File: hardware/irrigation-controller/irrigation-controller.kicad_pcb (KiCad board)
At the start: 2 copper layers, 109 x 48.3 mm, 39 parts, among them J1 RS485, J12 RELAY_2, J3 I/O, J5 RF Module, J6 PWR 24V, J7 RELAY_1, J8 ESP32, J9 ESP32, U1 AQY280EH, U3 AQY280EH, U4 TPS54331DR, U6 MAX3485

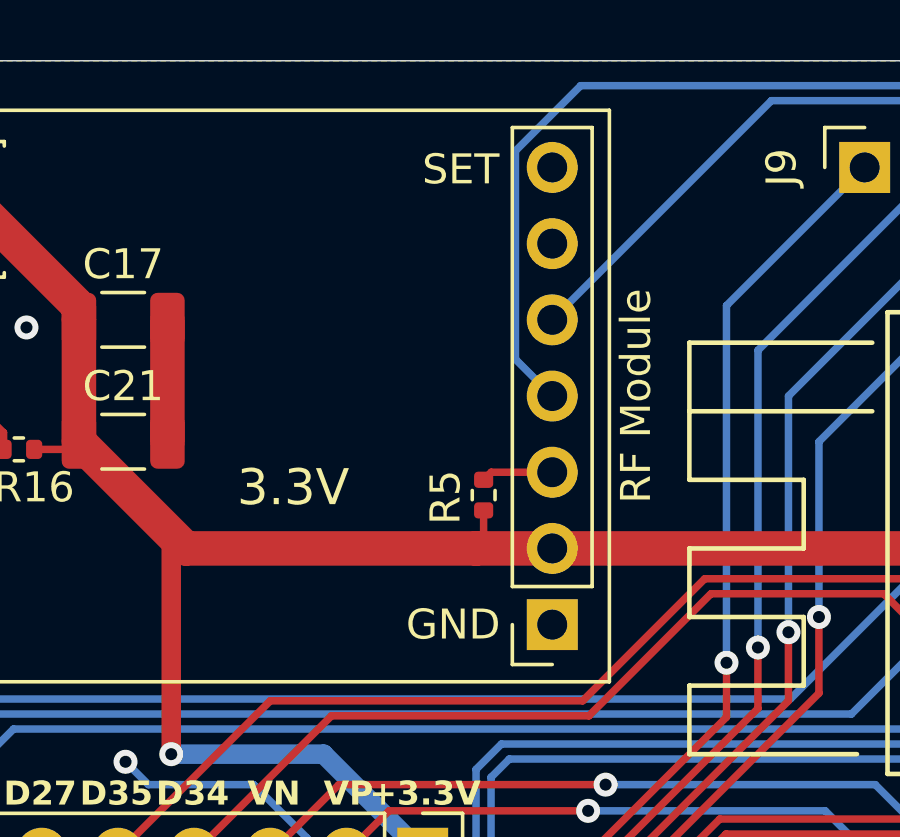
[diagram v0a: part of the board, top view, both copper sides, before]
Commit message: Update remote unit PCB
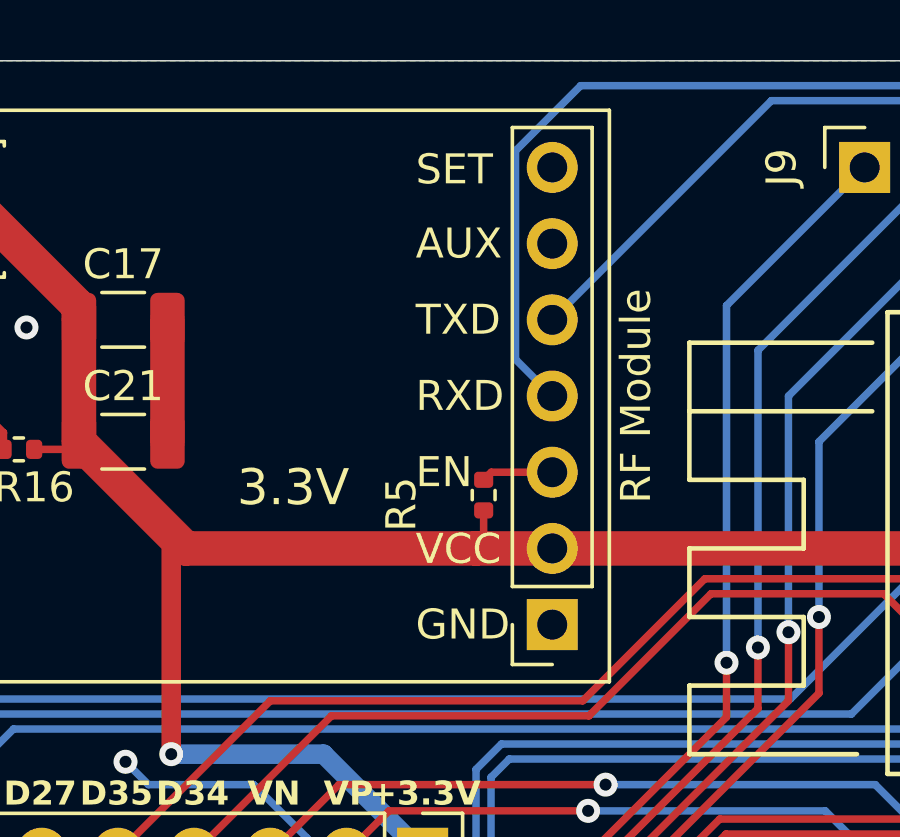
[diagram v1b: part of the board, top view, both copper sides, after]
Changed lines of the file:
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@@
     (property "ki_keywords" "connector")
     (attr through_hole)
-    (fp_text reference "J5" (at 0 -2.77) (layer "F.Fab")
-        (effects (font (size 1 1) (thickness 0.15)))
-    )
-    (fp_text value "RF Module" (at -2.794 7.62 90) (layer "F.SilkS")
-        (effects (font (size 1 1) (thickness 0.15)))
-    )
-    (fp_text user "SET" (at 3.048 15.1725) (layer "F.SilkS")
-        (effects (font (size 1 1) (thickness 0.15)))
-    )
-    (fp_text user "GND" (at 3.302 0) (layer "F.SilkS")
-        (effects (font (size 1 1) (thickness 0.15)))
-    )
-    (fp_text user "${REFERENCE}" (at 0 7.62 90) (layer "F.Fab")
+    (fp_text reference "J5" (at 0 -2.77 180) (layer "F.Fab")
+        (effects (font (size 1 1) (thickness 0.15)))
+    )
+    (fp_text value "RF Module" (at -2.794 7.62 -90) (layer "F.SilkS")
+        (effects (font (size 1 1) (thickness 0.15)))
+    )
+    (fp_text user "TXD" (at 4.552 10.16 180) (layer "F.SilkS")
+        (effects (font (size 1 1) (thickness 0.15)) (justify left))
+    )
+    (fp_text user "GND" (at 4.552 0 180) (layer "F.SilkS")
+        (effects (font (size 1 1) (thickness 0.15)) (justify left))
+    )
+    (fp_text user "AUX" (at 4.552 12.7 180) (layer "F.SilkS")
+        (effects (font (size 1 1) (thickness 0.15)) (justify left))
+    )
+    (fp_text user "VCC" (at 4.552 2.52 180) (layer "F.SilkS")
+        (effects (font (size 1 1) (thickness 0.15)) (justify left))
+    )
+    (fp_text user "SET" (at 4.552 15.1725 180) (layer "F.SilkS")
+        (effects (font (size 1 1) (thickness 0.15)) (justify left))
+    )
+    (fp_text user "RXD" (at 4.552 7.62 180) (layer "F.SilkS")
+        (effects (font (size 1 1) (thickness 0.15)) (justify left))
+    )
+    (fp_text user "EN" (at 4.552 5.08 180) (layer "F.SilkS")
+        (effects (font (size 1 1) (thickness 0.15)) (justify left))
+    )
+    (fp_text user "${REFERENCE}" (at 0 7.62 -90) (layer "F.Fab")
         (effects (font (size 1 1) (thickness 0.15)))
     )
@@
     (property "ki_keywords" "R res resistor")
     (attr smd)
-    (fp_text reference "R5" (at 0.072 1.27 90) (layer "F.SilkS")
-        (effects (font (size 1 1) (thickness 0.15)))
-    )
+    (fp_text reference "R5" (at 0.3048 2.7432 90) (layer "F.SilkS")
+        (effects (font (size 1 1) (thickness 0.15)))
+    )
